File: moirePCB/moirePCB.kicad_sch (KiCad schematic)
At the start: 53 parts, among them J1 USB_C_Receptacle, J2 Conn_01x06_Socket, SW3 SW_DPDT_x2, U1 ESP32-PICO-D4, U1 TLC555xD, U2 BQ24075RGT, U3 TLV73333PDBV, U4 RFM95W-915S2, U5 CH340E, U7 HDC1080, U8 AP2281-1WG-7, U9 AP2281-1WG-7, Y2 32.768kHz

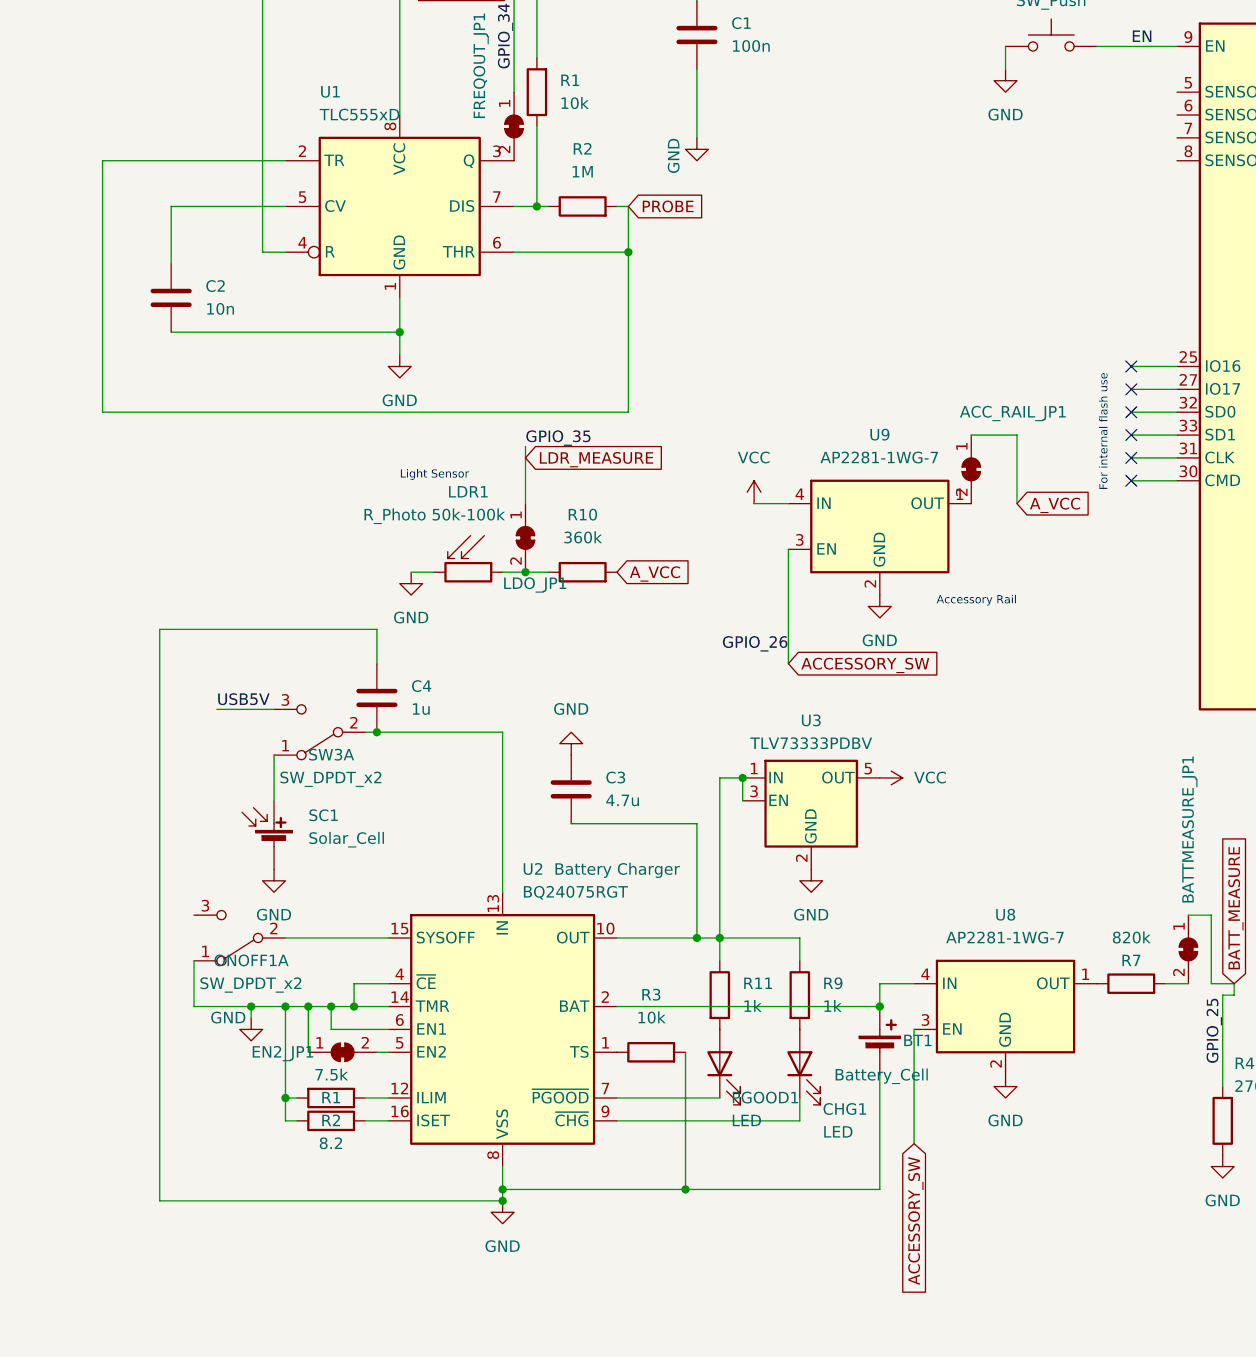
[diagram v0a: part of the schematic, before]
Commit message: bq25504
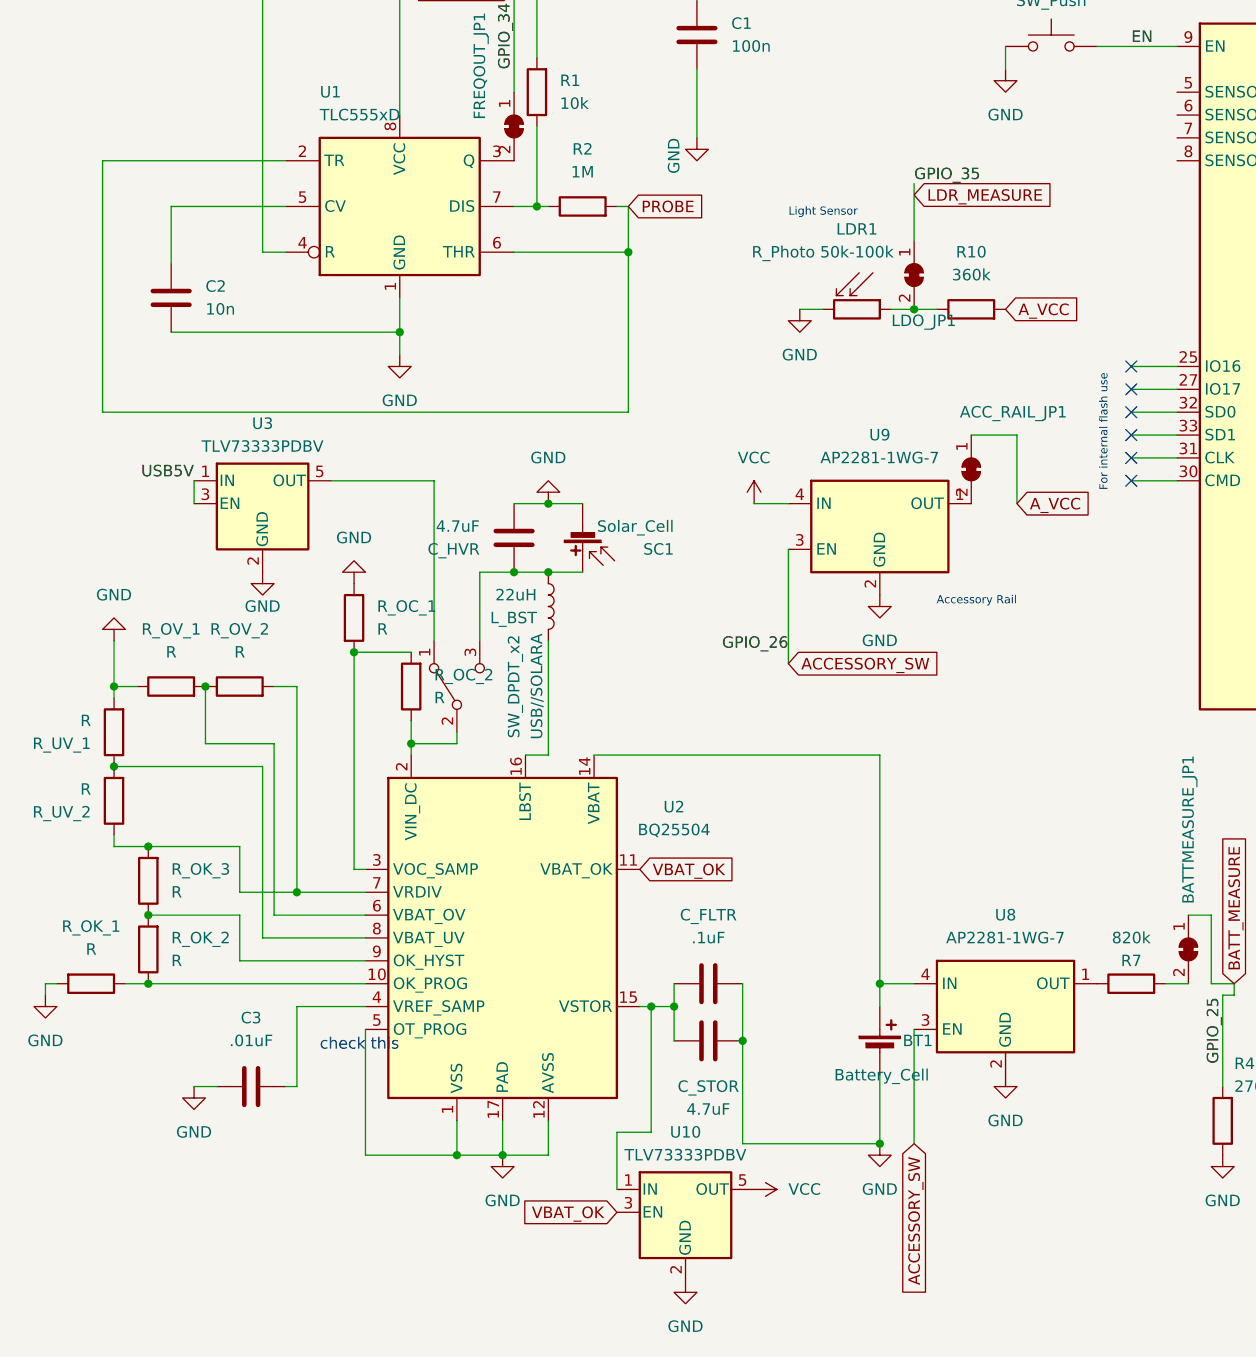
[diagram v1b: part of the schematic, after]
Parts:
- removed C4: 1u, Capacitor_SMD:C_0805_2012Metric, symbol Device:C
- removed CHG1, PGOOD1: LED, LED_SMD:LED_0805_2012Metric, symbol Device:LED
- removed EN2_JP1: SolderJumper_2_Bridged, Jumper:SolderJumper-2_P1.3mm_Bridged_RoundedPad1.0x1.5mm, symbol Jumper:SolderJumper_2_Bridged
- removed ONOFF1, SW3: SW_DPDT_x2, Button_Switch_SMD:SW_SPDT_PCM12, symbol Switch:SW_DPDT_x2
- removed R1: 7.5k, Resistor_SMD:R_0805_2012Metric, symbol Device:R
- removed R11, R9: 1k, Resistor_SMD:R_0805_2012Metric, symbol Device:R
- removed R2: 8.2, Resistor_SMD:R_0805_2012Metric, symbol Device:R
- removed R3: 10k, Resistor_SMD:R_0805_2012Metric, symbol Device:R
- removed U2: BQ24075RGT, Package_DFN_QFN:VQFN-16-1EP_3x3mm_P0.5mm_EP1.6x1.6mm, symbol Battery_Management:BQ24075RGT
- added C_FLTR: .1uF, symbol Device:C
- added C_HVR, C_STOR: 4.7uF, symbol Device:C
- added L_BST: 22uH, symbol Device:L
- added R_OC_1, R_OC_2, R_OK_1, R_OK_2, R_OK_3, R_OV_1, R_OV_2, R_UV_1, R_UV_2: R, symbol Device:R
- added U10: TLV73333PDBV, Package_TO_SOT_SMD:SOT-23-5, symbol Regulator_Linear:TLV73333PDBV
- added U2: BQ25504, Package_DFN_QFN:VQFN-16-1EP_3x3mm_P0.5mm_EP1.68x1.68mm, symbol Battery_Management:BQ25504
- added USB//SOLAR: SW_DPDT_x2, Button_Switch_SMD:SW_SPDT_PCM12, symbol Switch:SW_DPDT_x2
- C3: value 4.7u -> .01uF; footprint Capacitor_SMD:C_0805_2012Metric -> (none)
- SC1: footprint Connector_PinHeader_2.54mm:PinHeader_1x02_P2.54mm_Horizontal -> (none)
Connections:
- net GND: now also C_FLTR.2, C_HVR.2, C_STOR.1, R_OC_1.1, R_OK_1.2, R_OV_1.1, R_UV_1.2, U10.2 (GND), U2.1 (VSS), U2.12 (AVSS), U2.13 (VSS), U2.17 (PAD), U2.5 (OT_PROG)
- net IN: now also U10.5 (OUT), U2.14 (VBAT); no longer U3.5 (OUT)
- net USB5V: now also U3.1 (IN), U3.3 (EN)
- net at SC1.1 (+): now also C_HVR.1, L_BST.1, USB//SOLAR.3 (C)
- new net: U3.5 (OUT), USB//SOLAR.1 (A)
- new net: R_OK_1.1, R_OK_2.1, U2.10 (OK_PROG)
- new net: C_FLTR.1, C_STOR.2, U10.1 (IN), U2.15 (VSTOR)
- new net: L_BST.2, U2.16 (LBST)
- new net: R_OC_2.1, U2.2 (VIN_DC), USB//SOLAR.2 (B)
- new net: R_OC_1.2, R_OC_2.2, U2.3 (VOC_SAMP)
- new net: C3.2, U2.4 (VREF_SAMP)
- new net: R_OV_1.2, R_OV_2.1, U2.6 (VBAT_OV)
- new net: R_OK_3.2, R_OV_2.2, R_UV_2.1, U2.7 (VRDIV)
- new net: R_UV_1.1, R_UV_2.2, U2.8 (VBAT_UV)
- new net: R_OK_2.2, R_OK_3.1, U2.9 (OK_HYST)
- new net VBAT_OK: U10.3 (EN), U2.11 (VBAT_OK)
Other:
- note added: "check this"
- moved on the sheet: LDO_JP1, LDR1, R10
